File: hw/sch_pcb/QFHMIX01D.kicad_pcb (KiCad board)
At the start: 2 copper layers, 90.9 x 90.9 mm, 205 parts, among them J1 HEADER_1x08, J2 +9V, M1 HOLE, M2 HOLE, M3 HOLE, M4 HOLE, M5 HOLE, M6 HOLE, M7 HOLE, M8 HOLE, U1 NCP1117ST33, U11 TPS563249, U12 Si53322, U2 AD8343, U3 AD8343, U5 LT6604-10, U6 MPGA-105+, U7 MPGA-105+, U8 MGVA-63+, U9 MGVA-63+

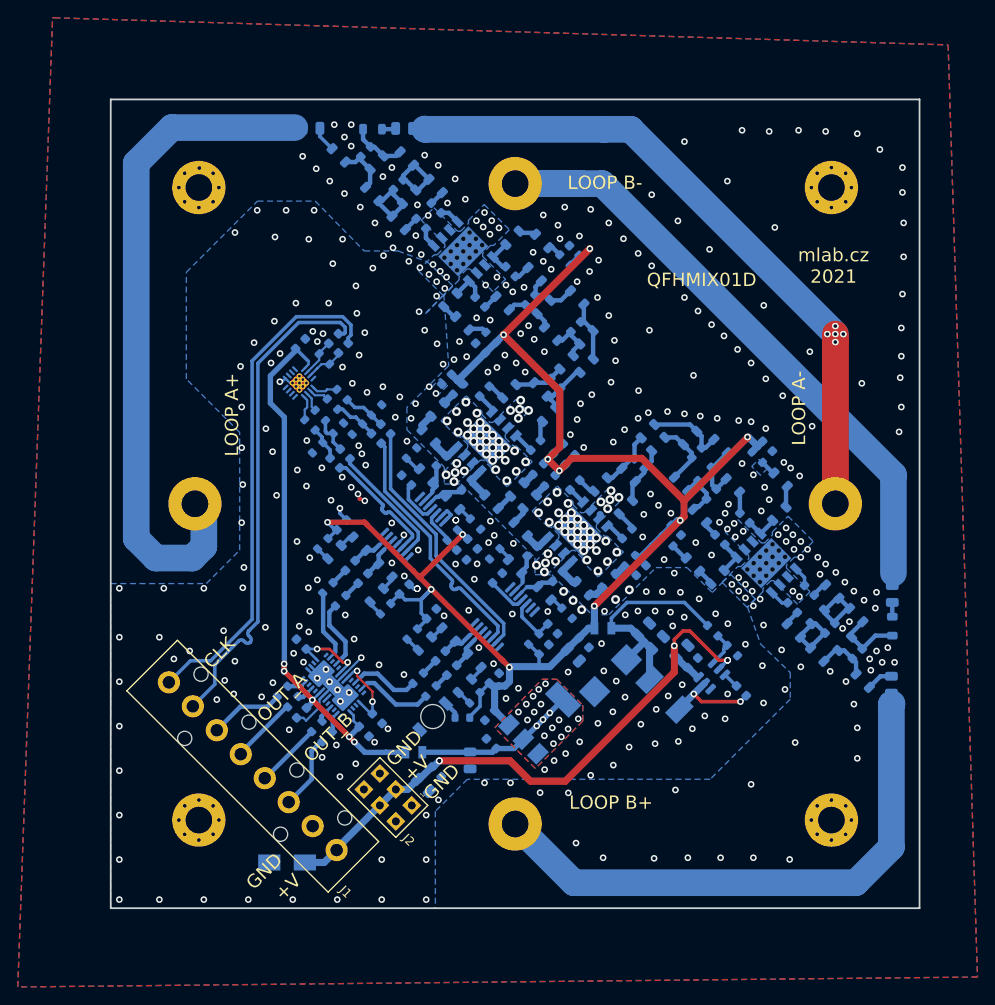
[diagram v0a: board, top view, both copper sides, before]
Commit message: Zmena pouzdra L 0805
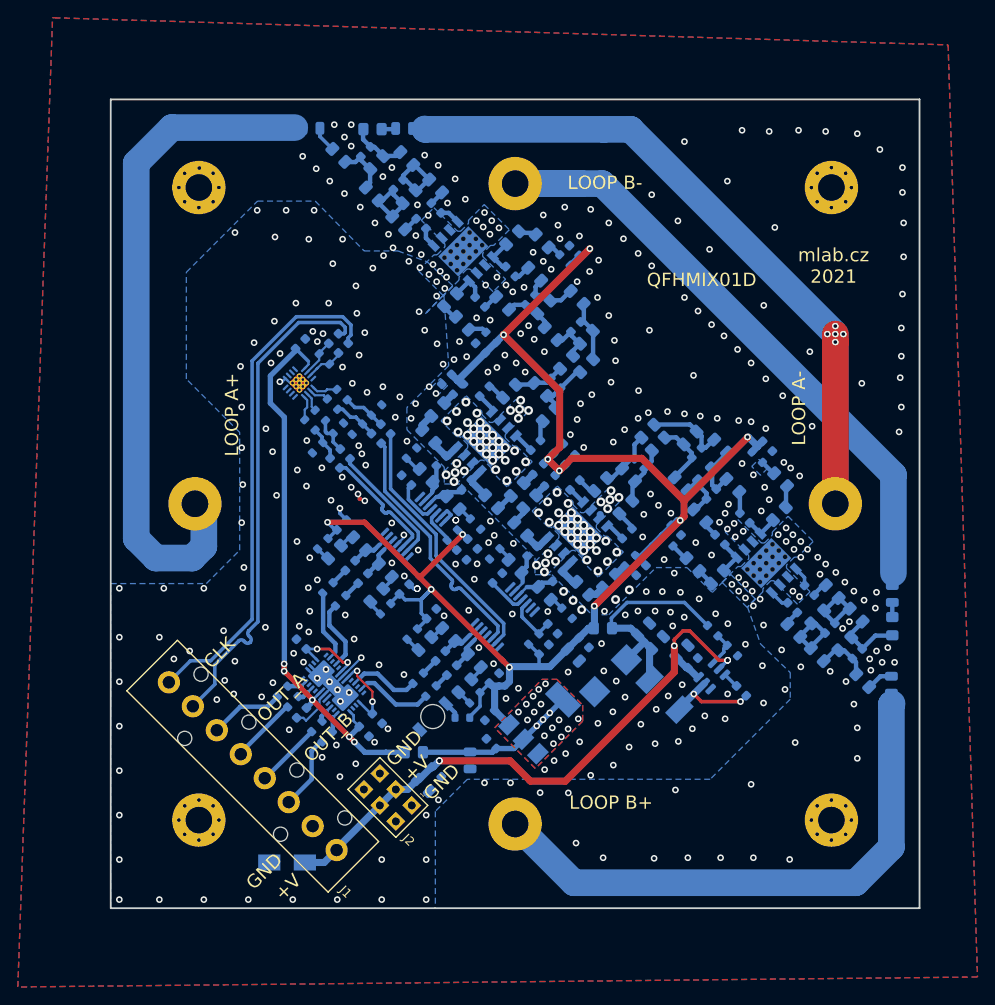
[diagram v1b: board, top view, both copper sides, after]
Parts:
- L1, L10, L11, L12, L13, L14, L15, L16, L17, L18, L19, L2, L20, L21, L22, L23, L24, L25, L26, L27, L28, L29, L3, L30, L31, L32, L33, L34, L35, L36, L37, L38, L39, L4, L40, L41, L42, L43, L44, L45, L46, L47, L5, L52, L53, L54, L55, L56, L57, L58, L59, L6, L60, L61, L62, L63, L64, L65, L66, L67, L68, L69, L7, L70, L8, L9: footprint Inductor_SMD:L_0805_2012Metric -> Inductor_SMD:L_0805_2012Metric_Pad1.15x1.40mm_HandSolder
- L48: footprint Mlab_L:SMD-0805 -> Inductor_SMD:L_0805_2012Metric_Pad1.15x1.40mm_HandSolder
- L51: footprint Mlab_R:SMD-0805 -> Inductor_SMD:L_0805_2012Metric_Pad1.15x1.40mm_HandSolder
